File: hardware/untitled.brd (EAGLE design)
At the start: 47 x 77.8 mm, 63 parts, among them J1 AUDIO_JACK_TRRSSMD_RA, J2 USB4110-GF-A, U1 AT32UC3A1512/1256/1128, U2 USD-SOCKETUSD, U3 LTC3558EUDTRPBFQFN-20_UD_LIT-M

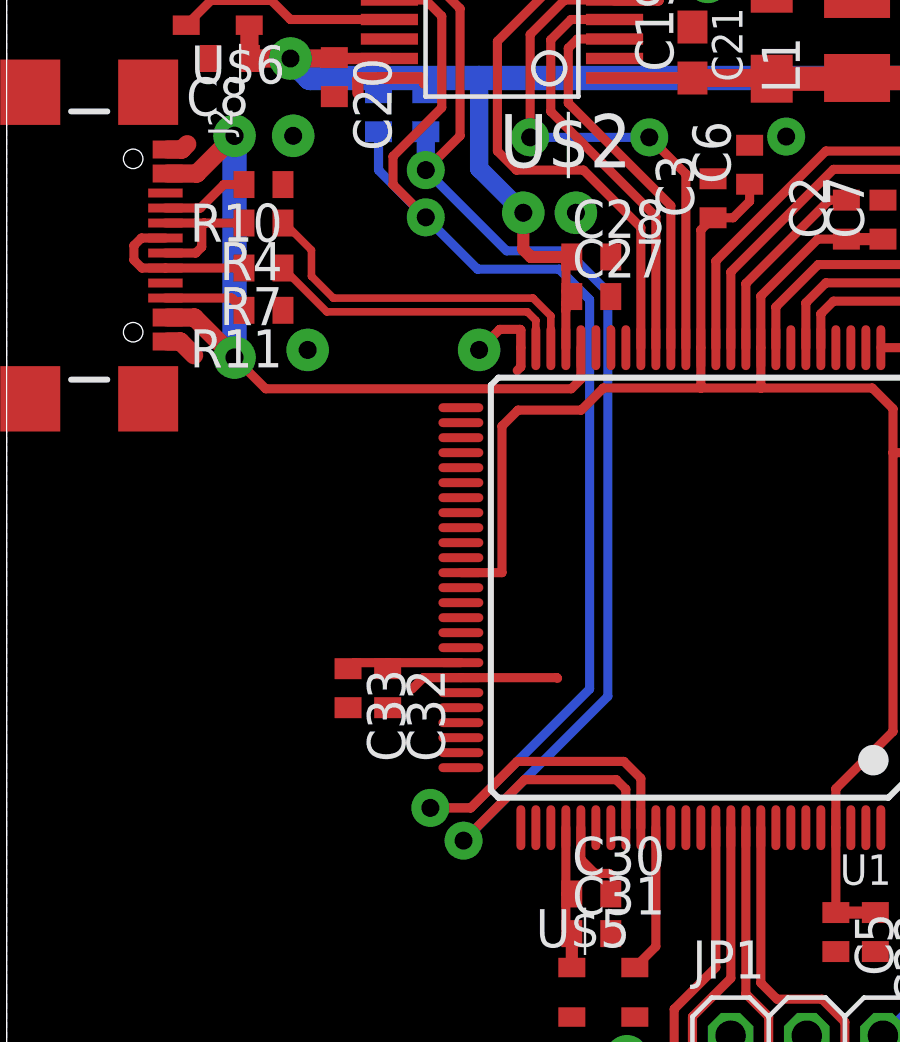
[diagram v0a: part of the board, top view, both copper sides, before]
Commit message: Minor update
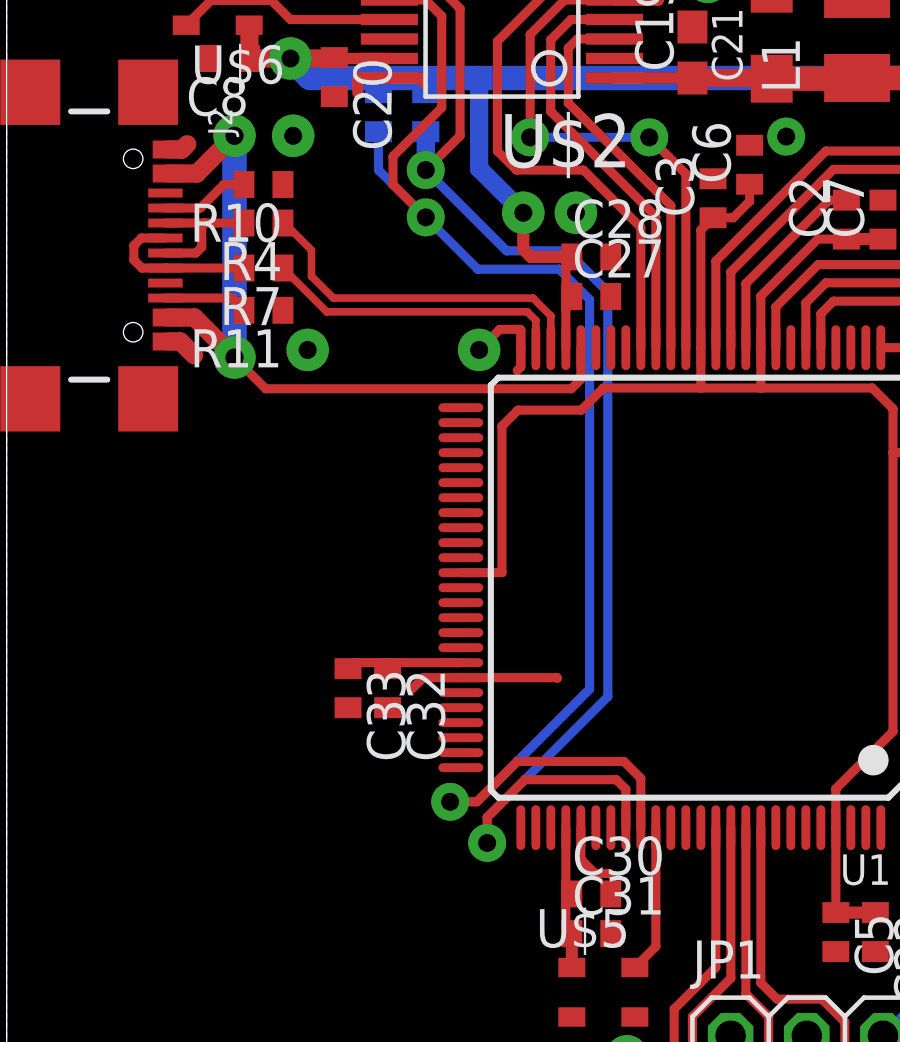
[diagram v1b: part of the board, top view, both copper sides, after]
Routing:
- net I2C1_SCL: track 49.4 -> 47.9 mm
- net I2C1_SDA: track 45.6 -> 45.1 mm
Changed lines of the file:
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@@
 <wire x1="21.1394" y1="25.4442" x2="20.574" y2="26.0096" width="0.3048" layer="1"/>
 <wire x1="20.574" y1="26.0096" x2="17.018" y2="26.0096" width="0.3048" layer="1"/>
-<wire x1="17.018" y1="26.0096" x2="15.4686" y2="24.4602" width="0.3048" layer="1"/>
-<via x="14.1224" y="24.4602" extent="1-16" drill="0.6" diameter="1.27" shape="octagon"/>
-<wire x1="14.1224" y1="24.4602" x2="15.4686" y2="24.4602" width="0.3048" layer="1"/>
-<wire x1="19.431" y1="28.4226" x2="15.4686" y2="24.4602" width="0.3048" layer="16"/>
-<wire x1="14.1224" y1="24.4602" x2="15.4686" y2="24.4602" width="0.3048" layer="16"/>
+<wire x1="17.018" y1="26.0096" x2="15.6718" y2="24.6634" width="0.3048" layer="1"/>
+<via x="14.7828" y="24.6634" extent="1-16" drill="0.6" diameter="1.27" shape="octagon"/>
 <wire x1="19.431" y1="41.402" x2="19.431" y2="28.4226" width="0.3048" layer="16"/>
 <wire x1="14.5034" y1="47.8028" x2="12.8778" y2="46.1772" width="0.3048" layer="1"/>
 <wire x1="12.8778" y1="46.1772" x2="12.8778" y2="45.2374" width="0.3048" layer="1"/>
-<wire x1="12.8778" y1="45.2374" x2="13.97" y2="44.1452" width="0.3048" layer="1"/>
+<wire x1="13.97" y1="44.1452" x2="12.8778" y2="45.2374" width="0.3048" layer="1"/>
 <wire x1="19.431" y1="41.402" x2="18.415" y2="42.418" width="0.3048" layer="16"/>
 <wire x1="18.415" y1="42.418" x2="15.6972" y2="42.418" width="0.3048" layer="16"/>
@@
 <wire x1="12.3952" y1="47.0004" x2="12.3952" y2="45.72" width="0.3048" layer="16"/>
 <wire x1="12.3952" y1="45.72" x2="13.97" y2="44.1452" width="0.3048" layer="16"/>
+<wire x1="14.7828" y1="24.6634" x2="15.6718" y2="24.6634" width="0.3048" layer="1"/>
+<wire x1="14.7828" y1="24.6634" x2="15.6718" y2="24.6634" width="0.3048" layer="16"/>
+<wire x1="15.6718" y1="24.6634" x2="17.018" y2="26.0096" width="0.3048" layer="16"/>
+<wire x1="17.018" y1="26.0096" x2="17.0688" y2="26.0604" width="0.3048" layer="16"/>
+<wire x1="19.431" y1="28.4226" x2="17.0688" y2="26.0604" width="0.3048" layer="16"/>
 </signal>
 <signal name="I2C1_SDA">
@@
 <wire x1="14.1778" y1="52.04" x2="15.113" y2="51.1048" width="0.3048" layer="1"/>
 <via x="13.97" y="45.72" extent="1-16" drill="0.6" diameter="1.27" shape="octagon"/>
-<via x="15.2292" y="23.368" extent="1-16" drill="0.6" diameter="1.27" shape="octagon"/>
+<via x="16.0166" y="23.2918" extent="1-16" drill="0.6" diameter="1.27" shape="octagon"/>
 <contactref element="R3" pad="1"/>
 <wire x1="20.6394" y1="23.8008" x2="20.6394" y2="25.0806" width="0.3048" layer="1"/>
 <wire x1="20.6394" y1="25.0806" x2="20.32" y2="25.4" width="0.3048" layer="1"/>
-<wire x1="20.32" y1="25.4" x2="17.2612" y2="25.4" width="0.3048" layer="1"/>
-<wire x1="17.2612" y1="25.4" x2="15.2292" y2="23.368" width="0.3048" layer="1"/>
-<wire x1="20.0406" y1="28.1794" x2="15.2292" y2="23.368" width="0.3048" layer="16"/>
-<wire x1="20.0406" y1="28.1794" x2="20.0406" y2="41.656" width="0.3048" layer="16"/>
+<wire x1="20.32" y1="25.4" x2="17.272" y2="25.4" width="0.3048" layer="1"/>
+<wire x1="20.0406" y1="28.1686" x2="20.0406" y2="41.656" width="0.3048" layer="16"/>
 <wire x1="15.113" y1="51.1048" x2="15.113" y2="46.863" width="0.3048" layer="1"/>
 <wire x1="15.113" y1="46.863" x2="13.97" y2="45.72" width="0.3048" layer="1"/>
@@
 <wire x1="18.669" y1="43.0276" x2="16.6624" y2="43.0276" width="0.3048" layer="16"/>
 <wire x1="16.6624" y1="43.0276" x2="13.97" y2="45.72" width="0.3048" layer="16"/>
+<wire x1="16.0166" y1="23.2918" x2="16.0166" y2="24.1446" width="0.3048" layer="16"/>
+<wire x1="20.0406" y1="28.1686" x2="16.0166" y2="24.1446" width="0.3048" layer="16"/>
+<wire x1="16.0166" y1="23.2918" x2="16.0166" y2="24.1446" width="0.3048" layer="1"/>
+<wire x1="16.0166" y1="24.1446" x2="17.272" y2="25.4" width="0.3048" layer="1"/>
 </signal>
 <signal name="A_3V">
@@
 <wire x1="17.6394" y1="39.8008" x2="17.6394" y2="40.71130625" width="0.254" layer="1"/>
 <wire x1="17.6394" y1="40.71130625" x2="17.35510625" y2="40.9956" width="0.254" layer="1"/>
-<wire x1="17.35510625" y1="40.9956" x2="10.6696" y2="40.9956" width="0.254" layer="1"/>
-<wire x1="10.6696" y1="40.9956" x2="9.2098" y2="42.4554" width="0.254" layer="1"/>
+<wire x1="10.6696" y1="40.9956" x2="17.35510625" y2="40.9956" width="0.254" layer="1"/>
+<wire x1="9.2098" y1="42.4554" x2="10.6696" y2="40.9956" width="0.254" layer="1"/>
 </signal>
 <signal name="D_N">
@@
 <wire x1="18.1394" y1="39.8008" x2="18.1394" y2="40.85789375" width="0.254" layer="1"/>
 <wire x1="18.1394" y1="40.85789375" x2="17.54449375" y2="41.4528" width="0.254" layer="1"/>
-<wire x1="17.54449375" y1="41.4528" x2="10.88969375" y2="41.4528" width="0.254" layer="1"/>
-<wire x1="10.88969375" y1="41.4528" x2="10.16" y2="42.18249375" width="0.254" layer="1"/>
+<wire x1="10.88969375" y1="41.4528" x2="17.54449375" y2="41.4528" width="0.254" layer="1"/>
+<wire x1="10.16" y1="42.18249375" x2="10.88969375" y2="41.4528" width="0.254" layer="1"/>
 <wire x1="10.16" y1="42.18249375" x2="10.16" y2="43.053" width="0.254" layer="1"/>
 <wire x1="10.16" y1="43.053" x2="9.2576" y2="43.9554" width="0.254" layer="1"/>
